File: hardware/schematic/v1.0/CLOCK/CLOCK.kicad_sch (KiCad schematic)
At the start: 105 parts, among them J1 Conn_Coaxial, J10 Conn_Coaxial, J11 USB_C_Receptacle_USB2.0_16P, J12 Conn_01x04_Socket, J13 Conn_01x10_Socket, J2 Conn_Coaxial, J3 Conn_Coaxial, J4 Conn_Coaxial, J5 Conn_Coaxial, J6 Conn_Coaxial, J7 Conn_Coaxial, J8 Conn_Coaxial, J9 Conn_Coaxial, U1 LMK5B12204, U2 LMK1C1102, U3 LMK1C1102, U4 TPS78633, U5 TPS78633, U6 OCXO-10M

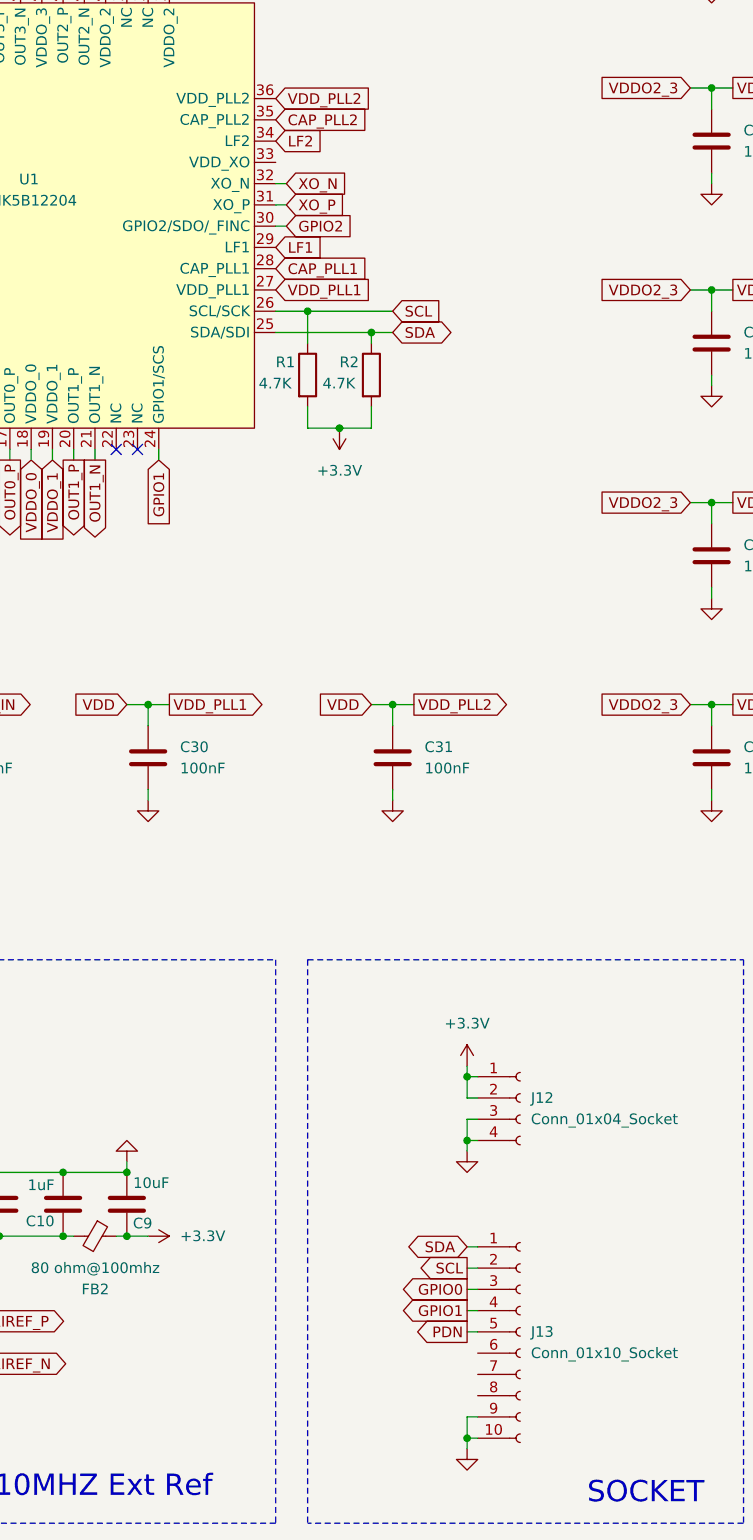
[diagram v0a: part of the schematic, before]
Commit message: sch update
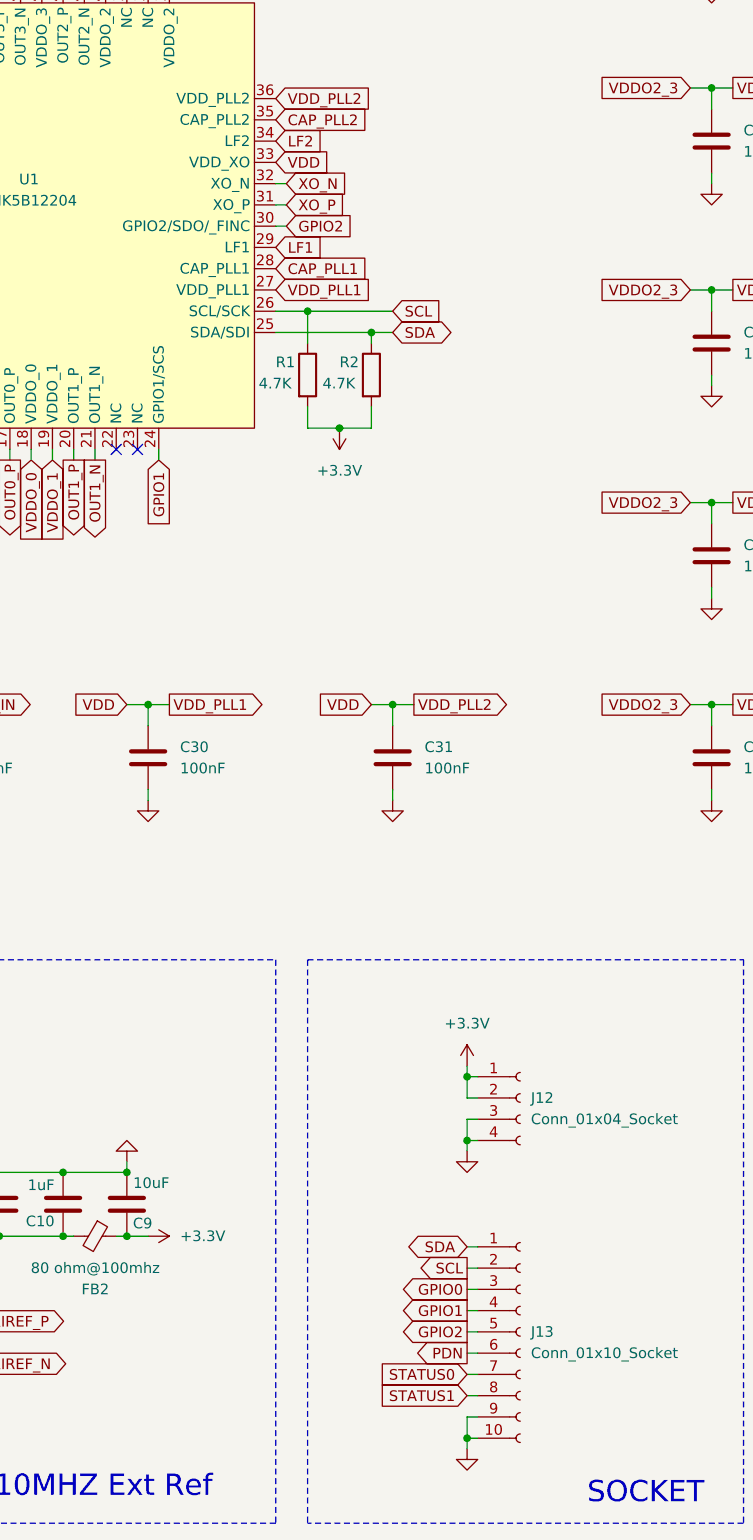
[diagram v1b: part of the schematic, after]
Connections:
- net GPIO2: now also J13.5 (Pin_5)
- net PDN: now also J13.6 (Pin_6); no longer J13.5 (Pin_5)
- net STATUS0: now also J13.7 (Pin_7)
- net STATUS1: now also J13.8 (Pin_8)
- net VDD: now also U1.33 (VDD_XO)
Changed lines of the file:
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@@
 	(wire
 		(pts
+			(xy 193.04 232.41) (xy 194.31 232.41)
+		)
+		(stroke
+			(width 0)
+			(type default)
+		)
+	)
+	(wire
+		(pts
 			(xy 293.37 113.03) (xy 306.07 113.03)
 		)
@@
 	(wire
 		(pts
+			(xy 193.04 234.95) (xy 194.31 234.95)
+		)
+		(stroke
+			(width 0)
+			(type default)
+		)
+	)
+	(wire
+		(pts
 			(xy 113.03 227.33) (xy 113.03 226.06)
 		)
@@
 	(wire
 		(pts
+			(xy 193.04 229.87) (xy 194.31 229.87)
+		)
+		(stroke
+			(width 0)
+			(type default)
+		)
+	)
+	(wire
+		(pts
 			(xy 125.73 31.75) (xy 125.73 33.02)
 		)
@@
 		)
 	)
+	(global_label "VDD"
+		(shape input)
+		(at 170.18 87.63 0)
+		(fields_autoplaced yes)
+		(effects
+			(font
+				(size 1.27 1.27)
+			)
+			(justify left)
+		)
+		(property "Intersheetrefs" "${INTERSHEET_REFS}"
+			(at 176.7938 87.63 0)
+			(hide yes)
+			(show_name no)
+			(do_not_autoplace no)
+			(effects
+				(font
+					(size 1.27 1.27)
+				)
+				(justify left)
+			)
+		)
+	)
 	(global_label "OUT2_N"
 		(shape input)
@@
 		)
 	)
+	(global_label "STATUS0"
+		(shape input)
+		(at 193.04 232.41 180)
+		(fields_autoplaced yes)
+		(effects
+			(font
+				(size 1.27 1.27)
+			)
+			(justify right)
+		)
+		(property "Intersheetrefs" "${INTERSHEET_REFS}"
+			(at 182.072 232.41 0)
+			(hide yes)
+			(show_name no)
+			(do_not_autoplace no)
+			(effects
+				(font
+					(size 1.27 1.27)
+				)
+				(justify right)
+			)
+		)
+	)
 	(global_label "VDDO_1"
 		(shape input)
@@
 		)
 	)
+	(global_label "PDN"
+		(shape output)
+		(at 193.04 229.87 180)
+		(fields_autoplaced yes)
+		(effects
+			(font
+				(size 1.27 1.27)
+			)
+			(justify right)
+		)
+		(property "Intersheetrefs" "${INTERSHEET_REFS}"
+			(at 186.1843 229.87 0)
+			(hide yes)
+			(show_name no)
+			(do_not_autoplace no)
+			(effects
+				(font
+					(size 1.27 1.27)
+				)
+				(justify right)
+			)
+		)
+	)
 	(global_label "VDD"
 		(shape output)
@@
 		)
 	)
+	(global_label "STATUS1"
+		(shape input)
+		(at 193.04 234.95 180)
+		(fields_autoplaced yes)
+		(effects
+			(font
+				(size 1.27 1.27)
+			)
+			(justify right)
+		)
+		(property "Intersheetrefs" "${INTERSHEET_REFS}"
+			(at 182.072 234.95 0)
+			(hide yes)
+			(show_name no)
+			(do_not_autoplace no)
+			(effects
+				(font
+					(size 1.27 1.27)
+				)
+				(justify right)
+			)
+		)
+	)
 	(global_label "CAP_DIG"
 		(shape input)
@@
 		)
 	)
-	(global_label "PDN"
+	(global_label "GPIO2"
 		(shape output)
 		(at 193.04 227.33 180)
@@
 		)
 		(property "Intersheetrefs" "${INTERSHEET_REFS}"
-			(at 186.1843 227.33 0)
+			(at 184.37 227.33 0)
 			(hide yes)
 			(show_name no)
